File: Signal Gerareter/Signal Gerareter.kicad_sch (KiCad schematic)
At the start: 10 parts, among them U1 LM324

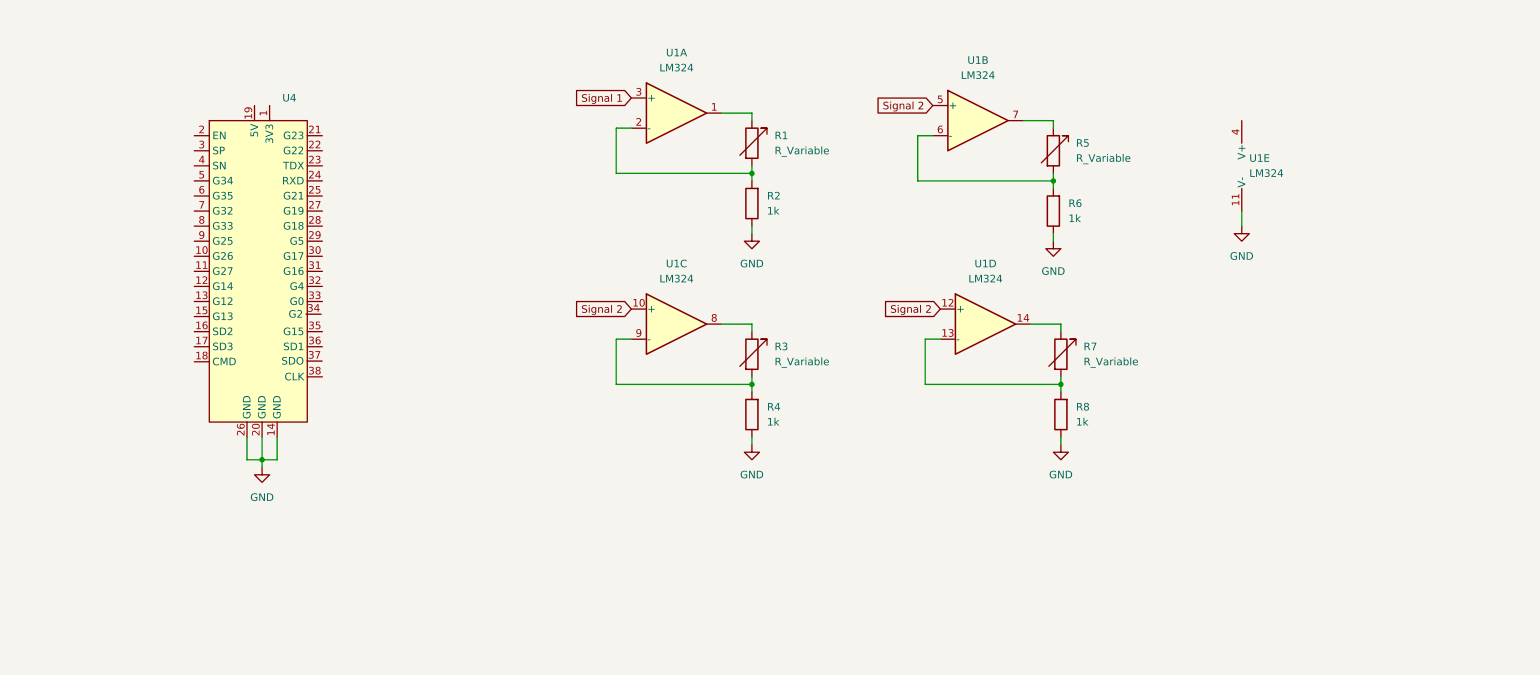
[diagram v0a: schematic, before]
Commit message: klein update
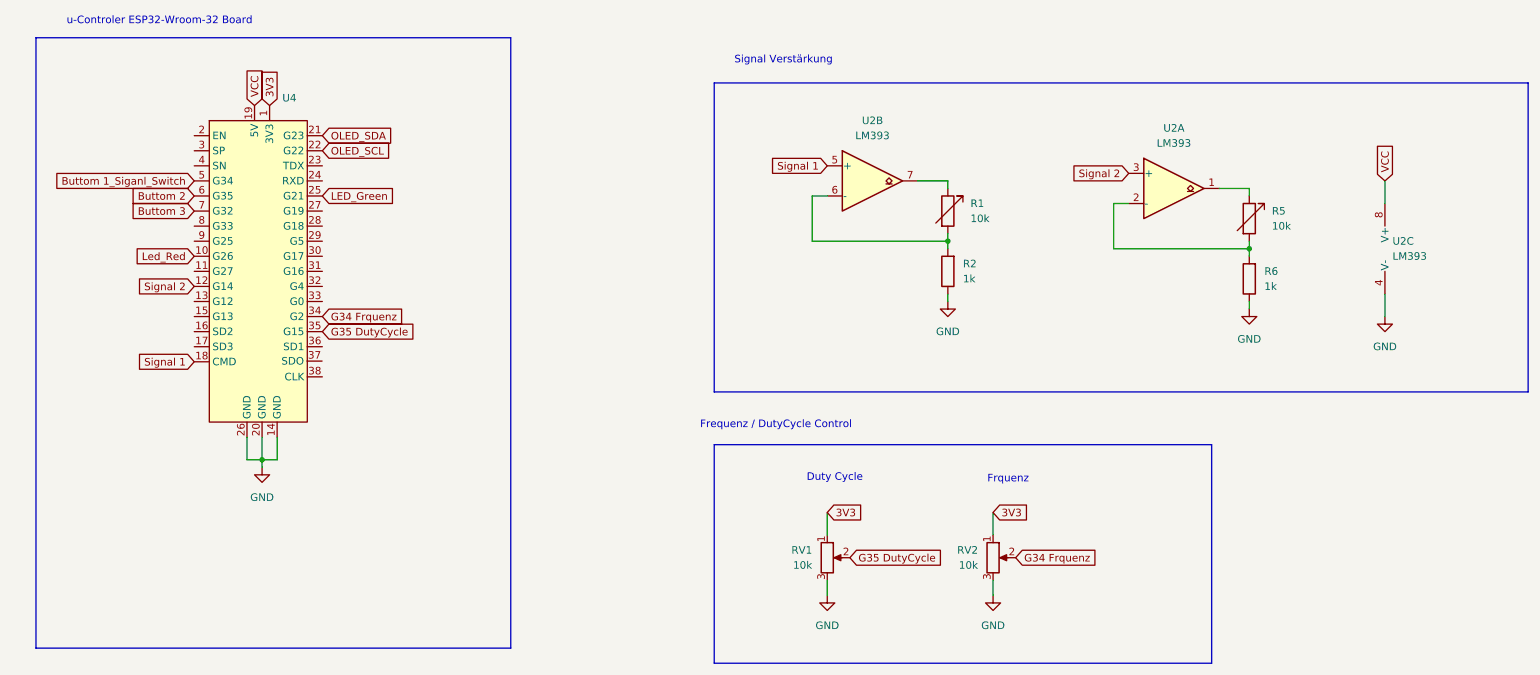
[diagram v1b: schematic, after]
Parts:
- removed R3, R7: R_Variable, Potentiometer_THT:Potentiometer_Alps_RK163_Single_Horizontal, symbol Device:R_Variable
- removed R4: 1k, Resistor_SMD:R_1206_3216Metric, symbol Device:R
- removed R8: 1k, Resistor_SMD:R_1210_3225Metric, symbol Device:R
- removed U1: LM324, Library:LM324_4, symbol Amplifier_Operational:LM324
- added RV1, RV2: 10k, symbol Device:R_Potentiometer
- added U2: LM393, symbol Comparator:LM393
- R1, R5: value R_Variable -> 10k
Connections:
- net GND: now also RV1.3, RV2.3, U2.4 (V-)
- net Signal 1: now also U4.18 (CMD), U2.5 (+)
- net Signal 2: now also U4.12 (G14), U2.3 (+)
- net at R1.1: now also U2.7
- net at R1.2, R2.2: now also U2.6 (-)
- net at R5.2, R6.2: now also U2.2 (-)
- net at R5.1: now also U2.1
- net 3V3: now reaches U4.1 (3V3)
- net 3V3: now also RV1.1, RV2.1
- net Led_Red: now reaches U4.10 (G26)
- net VCC: now reaches U4.19 (5V)
- net VCC: now also U2.8 (V+)
- net OLED_SDA: now reaches U4.21 (G23)
- net OLED_SCL: now reaches U4.22 (G22)
- net LED_Green: now reaches U4.25 (G21)
- net G34 Frquenz: now reaches U4.34 (G2)
- net G34 Frquenz: now also RV2.2
- net G35 DutyCycle: now reaches U4.35 (G15)
- net G35 DutyCycle: now also RV1.2
- net Buttom 1_Siganl_Switch: now reaches U4.5 (G34)
- net Buttom 2: now reaches U4.6 (G35)
- net Buttom 3: now reaches U4.7 (G32)
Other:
- note added: "Duty Cycle"
- note added: "Frequenz / DutyCycle Control"
- note added: "Frquenz"
- note added: "Signal Verstärkung"
- note added: "u-Controler ESP32-Wroom-32 Board"
- moved on the sheet: R1, R2, R5, R6
